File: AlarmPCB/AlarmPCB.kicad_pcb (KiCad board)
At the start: 2 copper layers, 96 x 56.9 mm, 13 parts

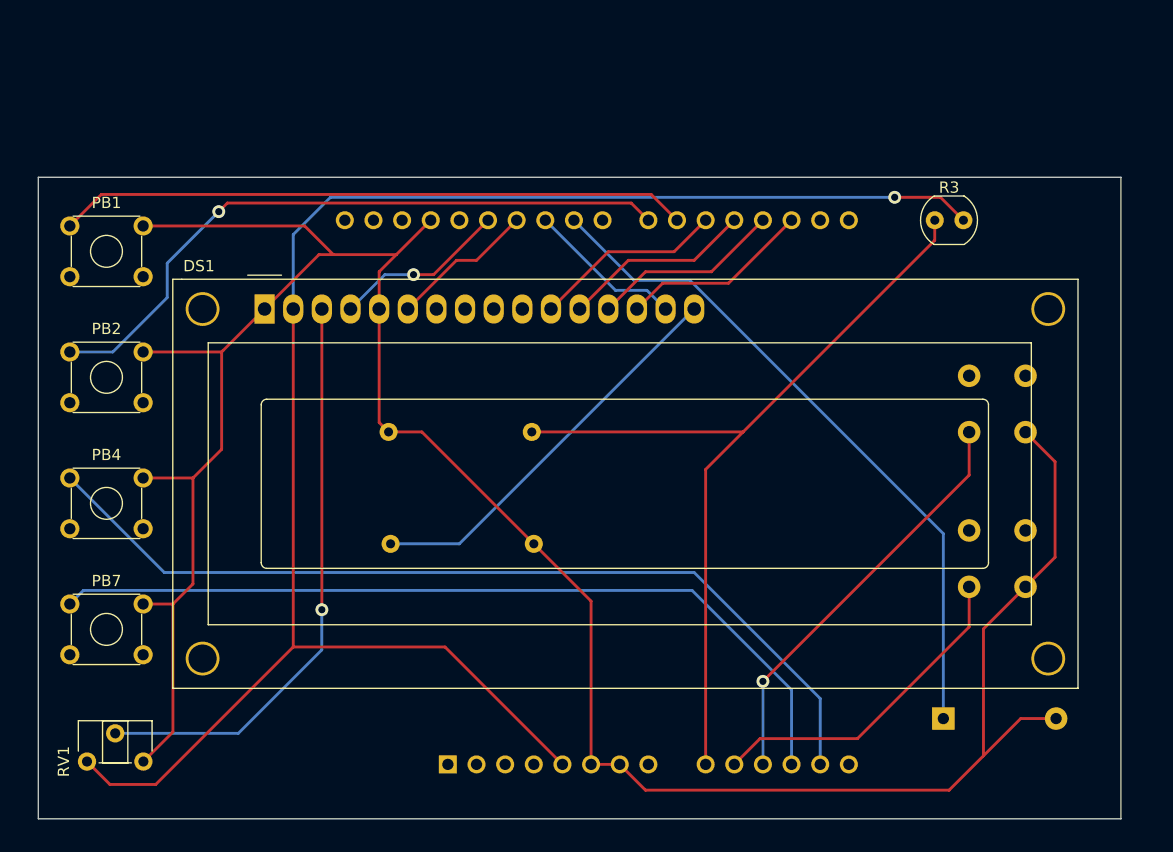
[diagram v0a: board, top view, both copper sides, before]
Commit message: Fixed Layout Issues
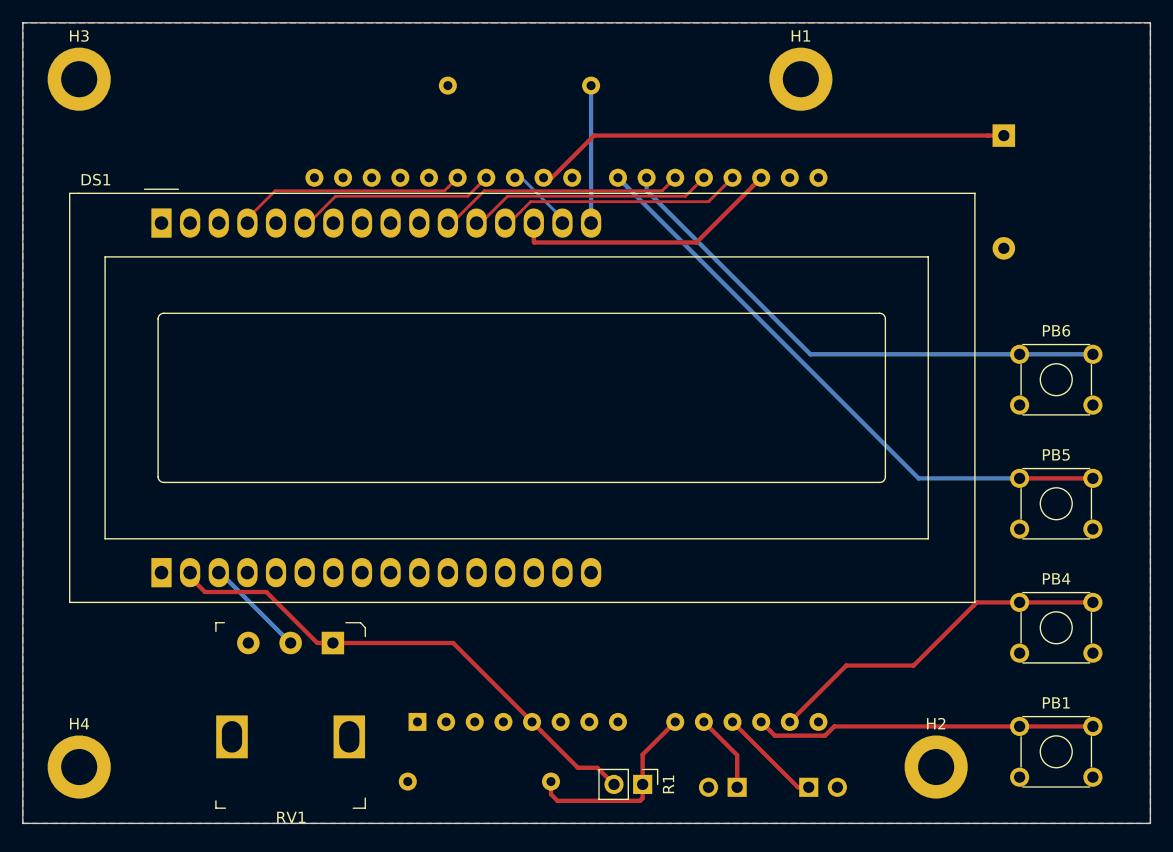
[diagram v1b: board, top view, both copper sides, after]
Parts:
- removed PB7: Backlight, Button_Switch_THT:SW_TH_Tactile_Omron_B3F-10xx
- added H1: MountingHole, MountingHole:MountingHole_3.2mm_M3_DIN965_Pad, F.Cu at (139.0, 99.0)
- added H2: MountingHole, MountingHole:MountingHole_3.2mm_M3_DIN965_Pad, F.Cu at (151.0, 160.0)
- added H3: MountingHole, MountingHole:MountingHole_3.2mm_M3_DIN965_Pad, F.Cu at (75.0, 99.0)
- added H4: MountingHole, MountingHole:MountingHole_3.2mm_M3_DIN965_Pad, F.Cu at (75.0, 160.0)
- added PB3: CancelAlarm, Connector_PinHeader_2.54mm:PinHeader_1x02_P2.54mm_Vertical, B.Cu at (133.3, 161.8)
- DS1: footprint Display:WC1602A -> ECE:WC1602A
- PB1: value Time+ -> Backlight; footprint Button_Switch_THT:SW_TH_Tactile_Omron_B3F-10xx -> ECE:SW_TH_Tactile
- PB2: value Time- -> Snooze; footprint Button_Switch_THT:SW_TH_Tactile_Omron_B3F-10xx -> Connector_PinHeader_2.54mm:PinHeader_1x02_P2.54mm_Vertical; moved to B.Cu
- PB4: footprint Button_Switch_THT:SW_TH_Tactile_Omron_B3F-10xx -> ECE:SW_TH_Tactile
- PB5: value CancelAlarm -> Time-; footprint Button_Switch_THT:Push_E-Switch_KS01Q01 -> ECE:SW_TH_Tactile; moved to F.Cu
- PB6: value Snooze -> Time+; footprint Button_Switch_THT:Push_E-Switch_KS01Q01 -> ECE:SW_TH_Tactile; moved to F.Cu
- R1: value 220R -> PhotoResistor; footprint Resistor_THT:R_Axial_DIN0309_L9.0mm_D3.2mm_P12.70mm_Horizontal -> Connector_PinHeader_2.54mm:PinHeader_1x02_P2.54mm_Vertical; moved to F.Cu
- R3: value PhotoResistor -> 220R; footprint OptoDevice:R_LDR_4.9x4.2mm_P2.54mm_Vertical -> Resistor_THT:R_Axial_DIN0309_L9.0mm_D3.2mm_P12.70mm_Horizontal; moved to B.Cu
- RV1: footprint Potentiometer_THT:Potentiometer_ACP_CA6-H2,5_Horizontal -> digikey-footprints:Potentiometer_P120PK-Y25BR10K
- moved PB1 95.2 mm to (158.4, 156.4)
- moved PB4 85.0 mm to (158.4, 145.4)
- moved PB2 76.1 mm to (139.7, 161.8), turned to 270 degrees
- moved BZ1 52.0 mm to (157.0, 104.0), turned to 270 degrees
- moved R3 32.7 mm to (120.4, 99.6), turned to 180 degrees
- moved R2 31.1 mm to (104.1, 161.3)
- moved R1 30.9 mm to (125.0, 161.5), turned to 270 degrees
- moved RV1 24.2 mm to (97.5, 149.0), turned to 180 degrees
- moved DS1 11.9 mm to (82.3, 111.8)
- moved PB5 10.6 mm to (158.4, 134.4)
- moved PB6 8.23 mm to (158.4, 123.4)
- moved A1 4.63 mm to (105.0, 156.0)
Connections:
- PB1 pad 1: /D6 -> /A3
- PB2 pad 1: /D7 -> /A2
- PB5 pad 1: /A1 -> /D7
- PB6 pad 1: /A2 -> /D6
- R1 pad 1: Net-(DS1-Pad16) -> Net-(A1-Pad9)
- R1 pad 2: GND -> +5V
- R3 pad 1: Net-(A1-Pad9) -> Net-(DS1-Pad16)
- R3 pad 2: +5V -> GND
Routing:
- net GND: track 227.1 -> 0.00 mm
- net +5V: track 150.6 -> 45.6 mm, vias 1 -> 0
- net Net-(A1-Pad9): track 75.4 -> 17.6 mm
- net /A4: track 80.5 -> 31.3 mm
- net /A3: track 74.8 -> 30.3 mm
- net Net-(DS1-Pad3): track 51.6 -> 8.96 mm, vias 1 -> 0
- net /A2: track 37.0 -> 9.16 mm, vias 1 -> 0
- net Net-(DS1-Pad16): track 35.6 -> 12.2 mm
- net /A1: track 29.4 -> 7.02 mm
- net Net-(A1-Pad24): track 60.7 -> 42.4 mm
- net /D6: track 56.0 -> 46.7 mm
- net /D10: track 13.9 -> 6.12 mm
- net /D2: track 17.0 -> 24.2 mm
- net /D7: track 59.2 -> 53.2 mm, vias 1 -> 0
- net /D12: track 15.5 -> 20.5 mm, vias 1 -> 0
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- added copper zone on B.Cu, net GND
- added copper zone on F.Cu, net GND
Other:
- board size 96 x 56.9 mm -> 100 x 71 mm
- rule trace_min: 0.254 -> 0.1
- rule via_min_size: 1.016 -> 0.2
